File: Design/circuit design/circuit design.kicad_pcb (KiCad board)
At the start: 2 copper layers, 37 parts, among them K1 R2_1A05, U1 STM32H7xx Dev Board, U2 ESP-01S, U3 HM-10, U4 uBlox_NEO_7M, U5 E-Paper_296x152_SSD1680, U6 MP1584EN, U7 EasyCard_IC, U8 TP4056

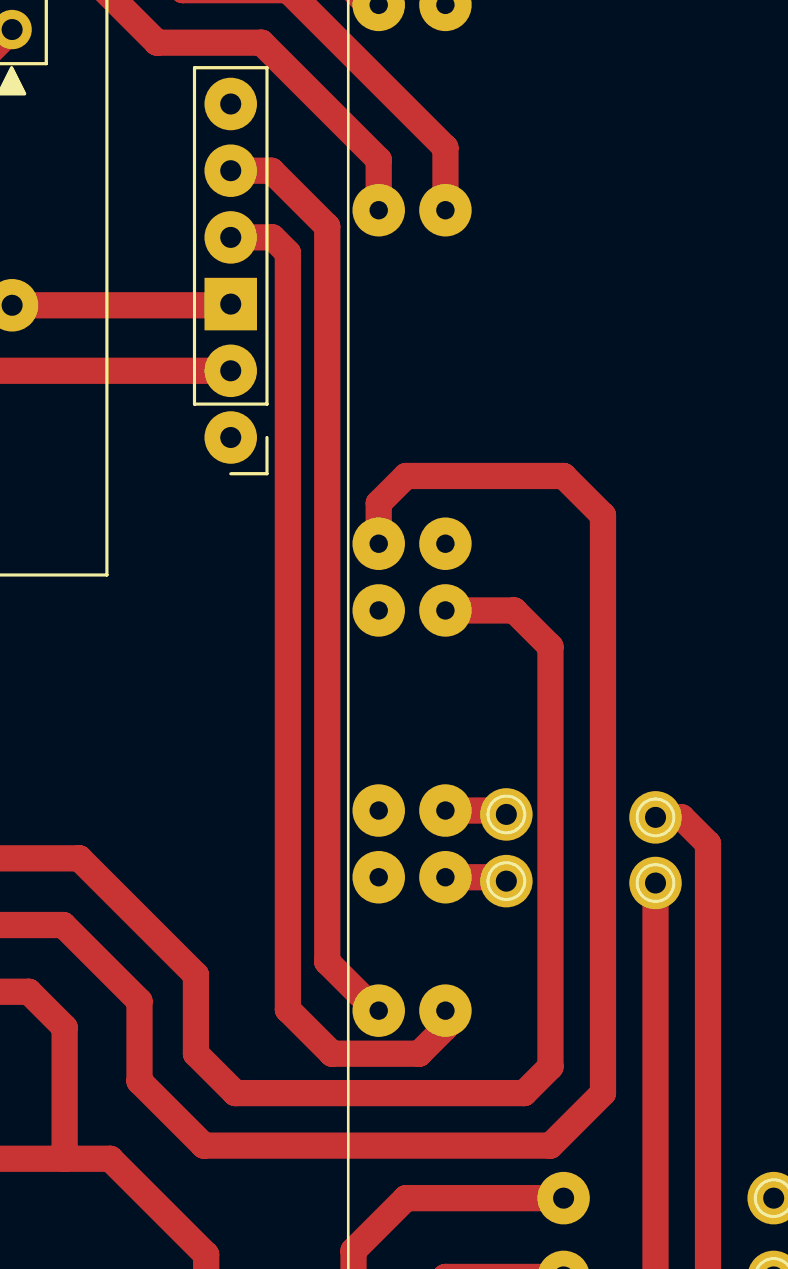
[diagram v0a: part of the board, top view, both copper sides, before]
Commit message: [2026-03-20 10:18:17 From Windows 11 Home]: Windows auto commit
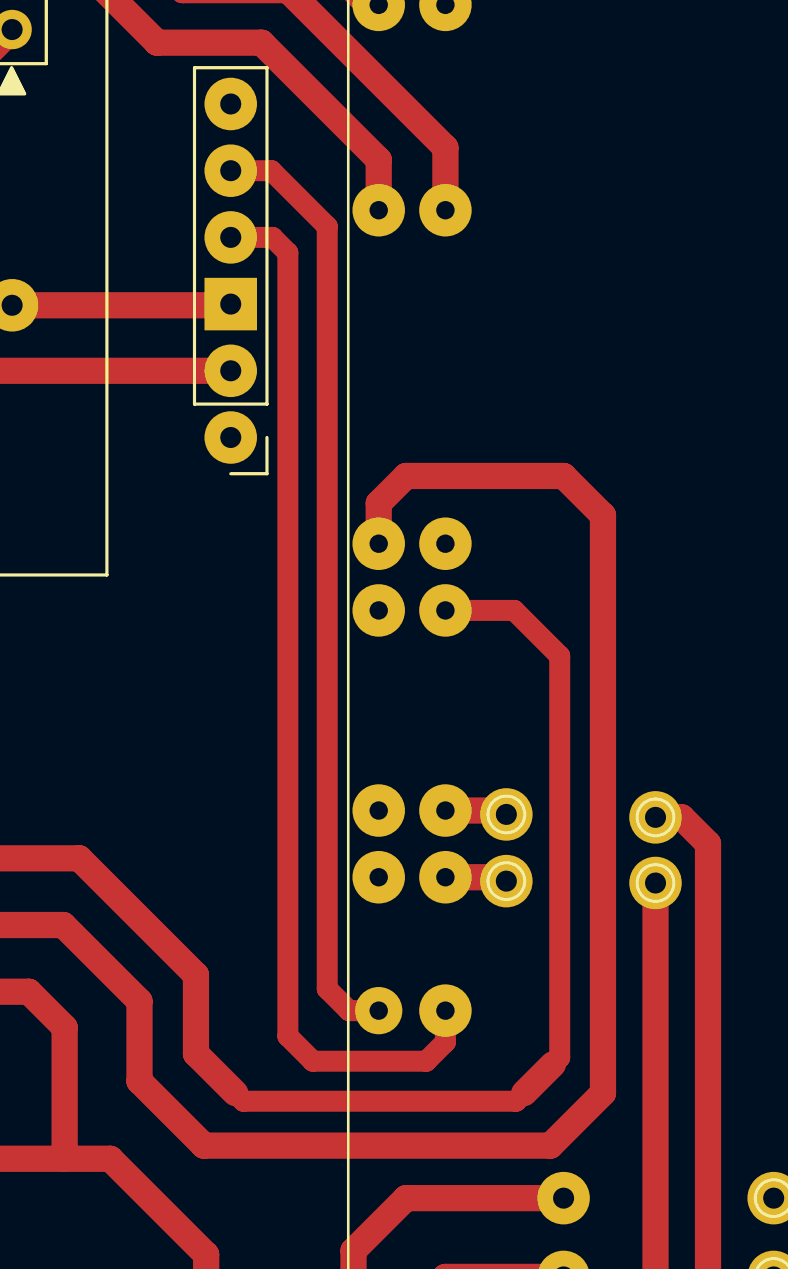
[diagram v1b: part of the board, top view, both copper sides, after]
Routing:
- net (no net): track 1042.3 -> 1044.6 mm
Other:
- board text added: "If you see this then the warranty is void"
- board text removed: "If you see this then warrenty void"
